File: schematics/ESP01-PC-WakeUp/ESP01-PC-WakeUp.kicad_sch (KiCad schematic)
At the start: 14 parts

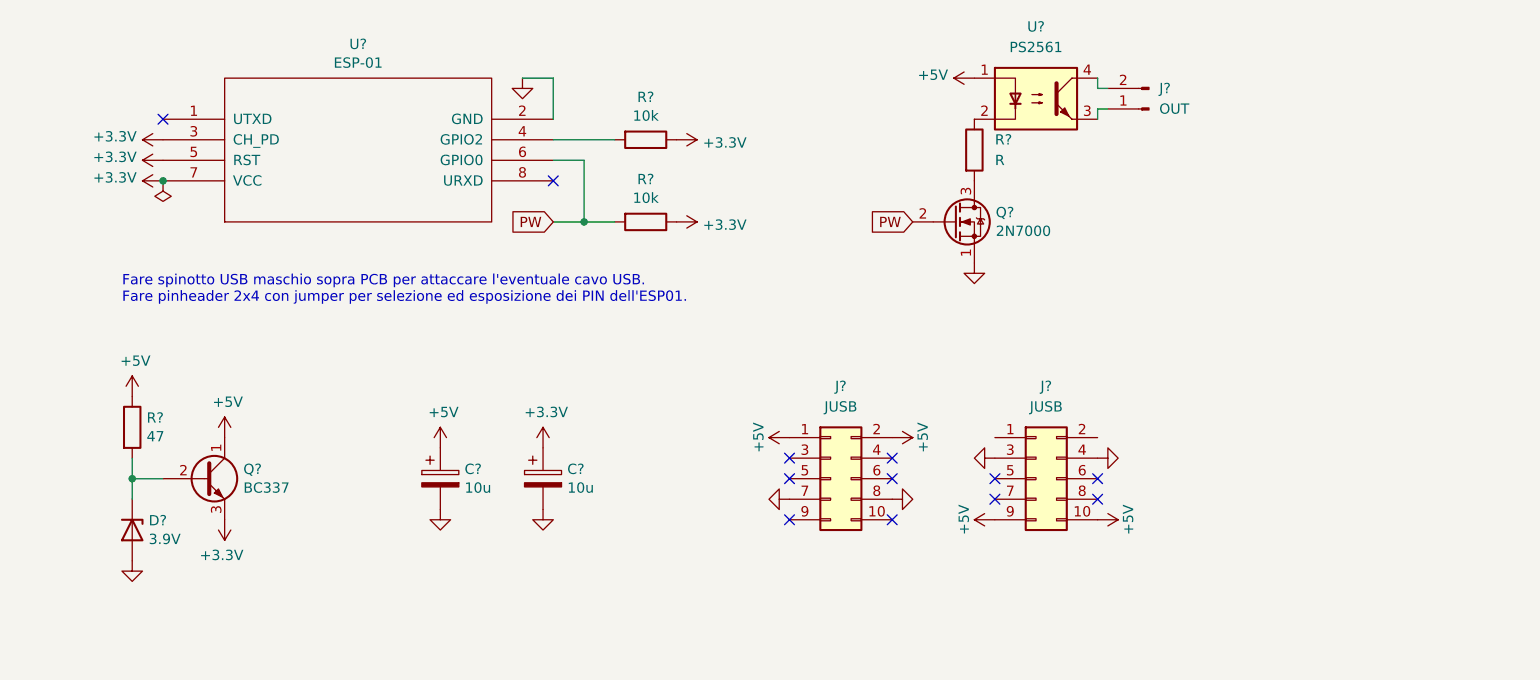
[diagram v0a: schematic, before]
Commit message: feat: shematics and footprints
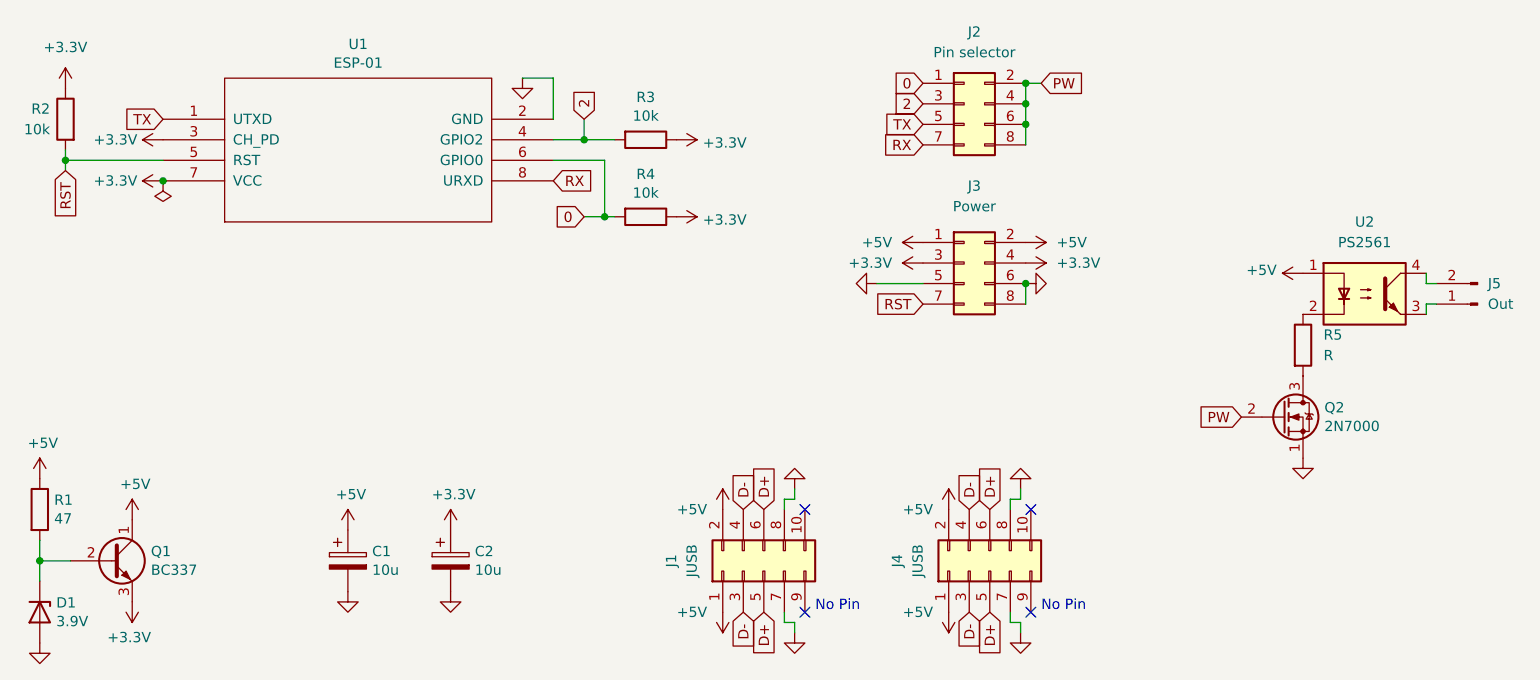
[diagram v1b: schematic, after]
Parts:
- removed J?: JUSB, Connector_PinHeader_2.54mm:PinHeader_2x05_P2.54mm_Vertical, symbol Connector_Generic:Conn_02x05_Odd_Even
- added J2: Pin selector, Connector_PinHeader_2.54mm:PinHeader_2x04_P2.54mm_Vertical, symbol Connector_Generic:Conn_02x04_Odd_Even
- added J3: Power, Connector_PinHeader_2.54mm:PinHeader_2x04_P2.54mm_Vertical, symbol Connector_Generic:Conn_02x04_Odd_Even
- added J4: JUSB, Connector_PinHeader_2.54mm:PinHeader_2x05_P2.54mm_Vertical, symbol Connector_Generic:Conn_02x05_Odd_Even
- added R2: 10k, Resistor_THT:R_Axial_DIN0207_L6.3mm_D2.5mm_P7.62mm_Horizontal, symbol Device:R
- C1, C2: renamed from C?; footprint Capacitor_THT:CP_Radial_D8.0mm_P3.50mm -> Capacitor_THT:CP_Radial_D4.0mm_P1.50mm
- J5: renamed from J?; value OUT -> Out; footprint (none) -> Connector_PinHeader_2.54mm:PinHeader_1x02_P2.54mm_Horizontal
- R5: renamed from R?; footprint (none) -> Resistor_THT:R_Axial_DIN0207_L6.3mm_D2.5mm_P7.62mm_Horizontal
- U2: renamed from U?; footprint Package_DIP:DIP-4_W7.62mm -> Package_DIP:DIP-4_W10.16mm
- gave numbers to parts that had none: 8
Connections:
- net +3V3: now also J3.3 (Pin_3), J3.4 (Pin_4), R2.1; no longer U1.5 (RST)
- net +5V: now also J3.1 (Pin_1), J3.2 (Pin_2), J4.1 (Pin_1), J4.2 (Pin_2)
- net GND: now also J3.5 (Pin_5), J3.6 (Pin_6), J3.8 (Pin_8), J4.7 (Pin_7), J4.8 (Pin_8)
- net PW: now also J2.2 (Pin_2), J2.4 (Pin_4), J2.6 (Pin_6), J2.8 (Pin_8); no longer R4.2, U1.6 (GPIO0)
- net 2: now reaches R3.2, U1.4 (GPIO2)
- net 2: now also J2.3 (Pin_3)
- net D-: now reaches J1.3 (Pin_3)
- net D-: now also J1.4 (Pin_4), J4.3 (Pin_3), J4.4 (Pin_4)
- net D+: now reaches J1.5 (Pin_5)
- net D+: now also J1.6 (Pin_6), J4.5 (Pin_5), J4.6 (Pin_6)
- net TX: now reaches U1.1 (UTXD)
- net TX: now also J2.5 (Pin_5)
- net RX: now reaches U1.8 (URXD)
- net RX: now also J2.7 (Pin_7)
- new net 0: J2.1 (Pin_1), R4.2, U1.6 (GPIO0)
- new net RST: J3.7 (Pin_7), R2.2, U1.5 (RST)
- no-connect marks 12 -> 4
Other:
- note added: "No Pin"
- note removed: "Fare spinotto USB maschio sopra PCB per attaccare l'eventuale cavo USB. Fare pinheader 2x4 con jumper per selezione ed esposizione dei PIN dell'ESP01."
- moved on the sheet: C1, C2, D1, J1, J5, Q1, Q2, R1, R4, R5, U2
